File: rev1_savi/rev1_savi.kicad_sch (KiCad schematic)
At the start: 5 parts, among them J1 Raspberry_Pi_4, U2 ICM-20948, U4 TFmini_S Lidar

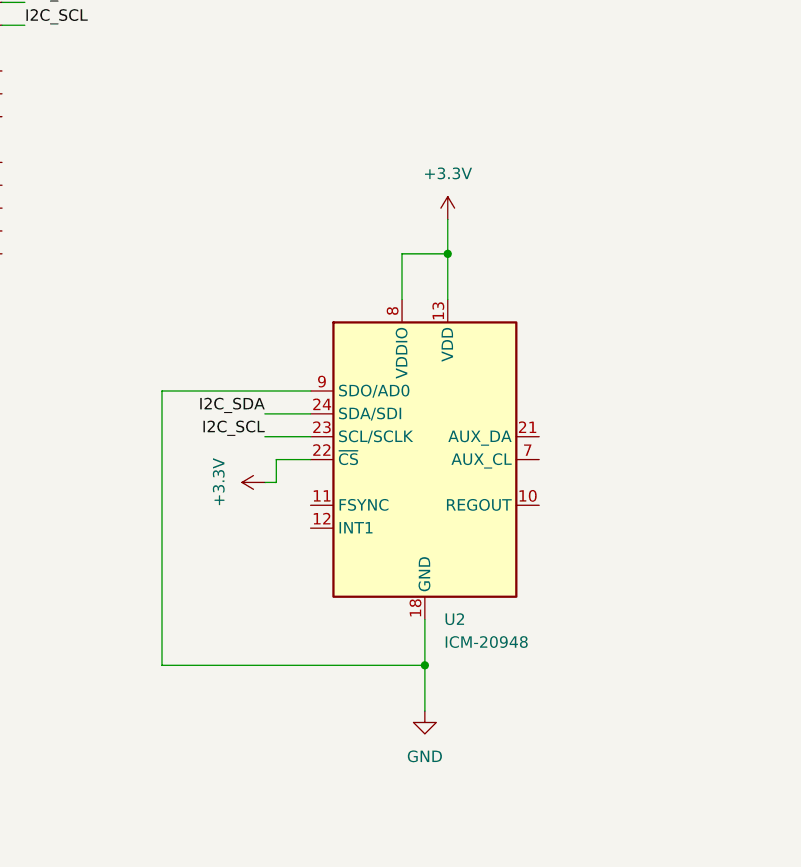
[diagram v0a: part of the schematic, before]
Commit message: Add files via upload
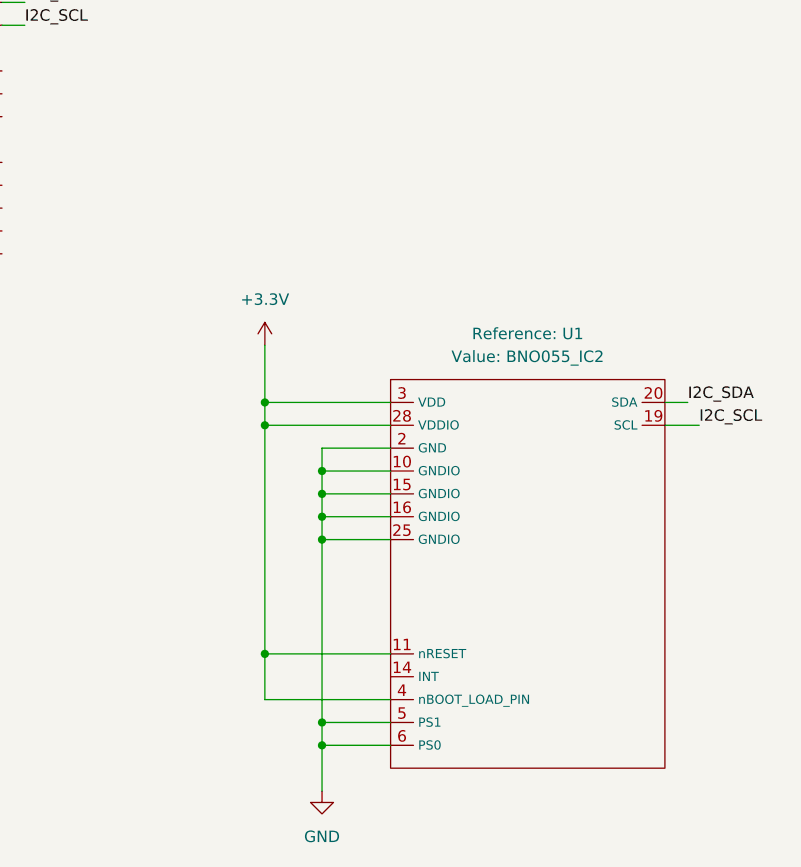
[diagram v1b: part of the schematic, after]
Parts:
- removed U2: ICM-20948, Sensor_Motion:InvenSense_QFN-24_3x3mm_P0.4mm, symbol Sensor_Motion:ICM-20948
- added U1: BNO055_IC2, symbol sensors:BNO055_IC2
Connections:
- net +3.3V: now also U1.11 (nRESET), U1.28 (VDDIO), U1.3 (VDD), U1.4 (nBOOT_LOAD_PIN)
- net GND: now also U1.10 (GNDIO), U1.15 (GNDIO), U1.16 (GNDIO), U1.2 (GND), U1.25 (GNDIO), U1.5 (PS1), U1.6 (PS0)
- net I2C_SCL: now also U1.19 (SCL)
- net I2C_SDA: now also U1.20 (SDA)
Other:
- title: SAVI I2C Sensor Bus (Pi + LiDAR + ICM-20948) -> SAVI I2C Sensor Bus (Pi + LiDAR + BNO055)
